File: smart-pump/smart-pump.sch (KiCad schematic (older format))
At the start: 19 parts, among them J1 Screw_Terminal_01x04, Q1 BC337, Q2 IRF5305, SW1 SW_SPST, U1 AZ1117-5.0, U2 Arduino_Pro_Mini

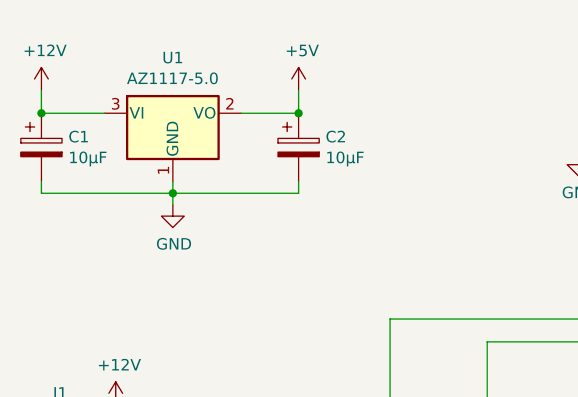
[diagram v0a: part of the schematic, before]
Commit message: Updated smart-pump
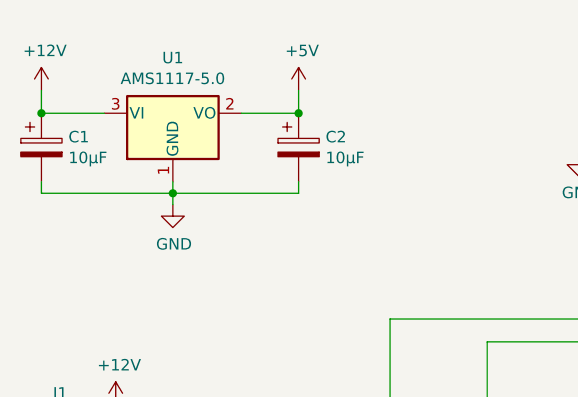
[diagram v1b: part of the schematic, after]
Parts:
- removed U1: AZ1117-5.0, symbol Regulator_Linear:AZ1117-5.0
- added U1: AMS1117-5.0, Package_TO_SOT_SMD:SOT-223-3_TabPin2, symbol Regulator_Linear:AMS1117-5.0
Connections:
- net +12V: now also U1.3 (VI)
- net +5V: now also U1.2 (VO)
- net GND: now also U1.1 (GND)
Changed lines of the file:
@@
-$EndComp
-$Comp
-L Regulator_Linear:AZ1117-5.0 U1
-U 1 1 624A95B3
-P 1725 1325
-F 0 "U1" H 1725 1567 50  0000 C CNN
-F 1 "AZ1117-5.0" H 1725 1476 50  0000 C CNN
-F 2 "" H 1725 1575 50  0001 C CIN
-F 3 "https://www.diodes.com/assets/Datasheets/AZ1117.pdf" H 1725 1325 50  0001 C CNN
-	1    1725 1325
-	1    0    0    -1
 $EndComp
 $Comp
@@
 Wire Wire Line
 	3725 1225 3725 1525
+$Comp
+L Regulator_Linear:AMS1117-5.0 U1
+U 1 1 6259A42F
+P 1725 1325
+F 0 "U1" H 1725 1567 50  0000 C CNN
+F 1 "AMS1117-5.0" H 1725 1476 50  0000 C CNN
+F 2 "Package_TO_SOT_SMD:SOT-223-3_TabPin2" H 1725 1525 50  0001 C CNN
+F 3 "http://www.advanced-monolithic.com/pdf/ds1117.pdf" H 1825 1075 50  0001 C CNN
+	1    1725 1325
+	1    0    0    -1
+$EndComp
 $EndSCHEMATC
